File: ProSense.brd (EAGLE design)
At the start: 25.4 x 36.7 mm, 26 parts, among them U2 LPC1114FHI33/303, U4 MIC2505 3.3

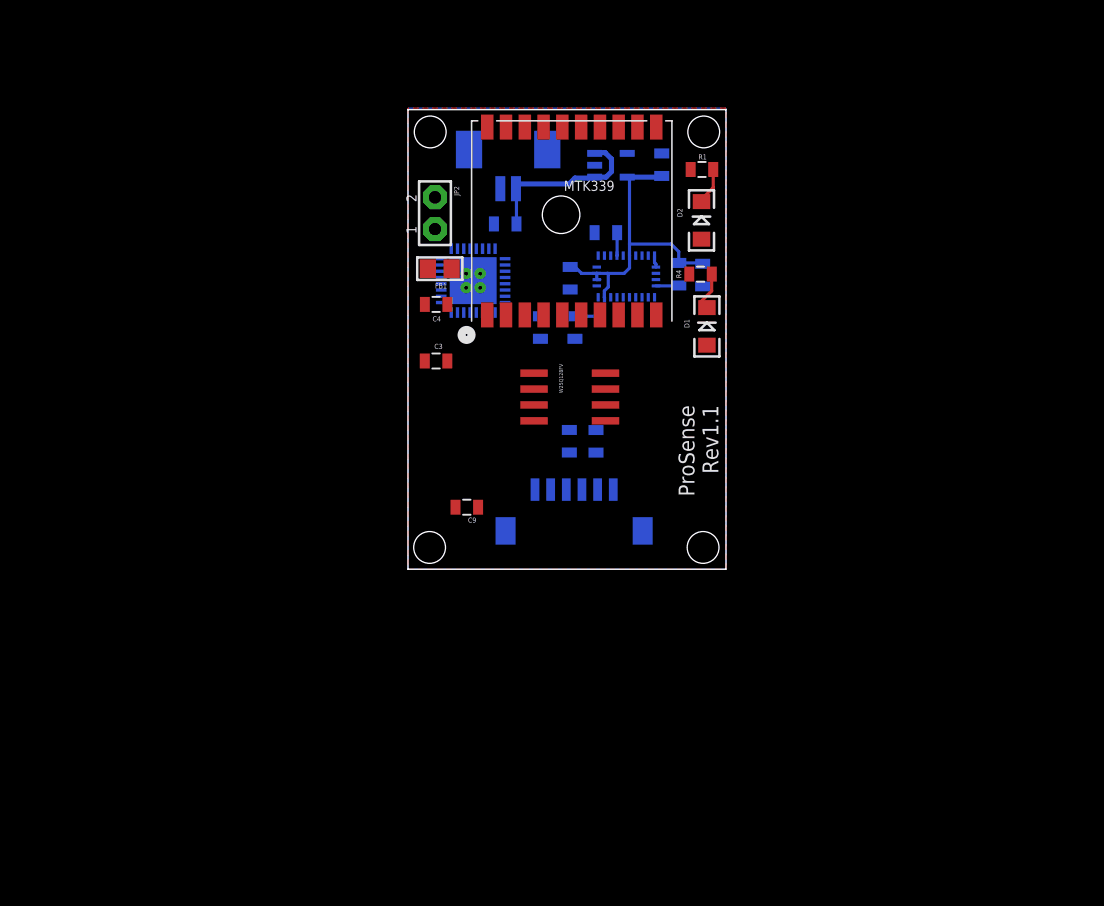
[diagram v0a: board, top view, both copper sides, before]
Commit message: Fixup
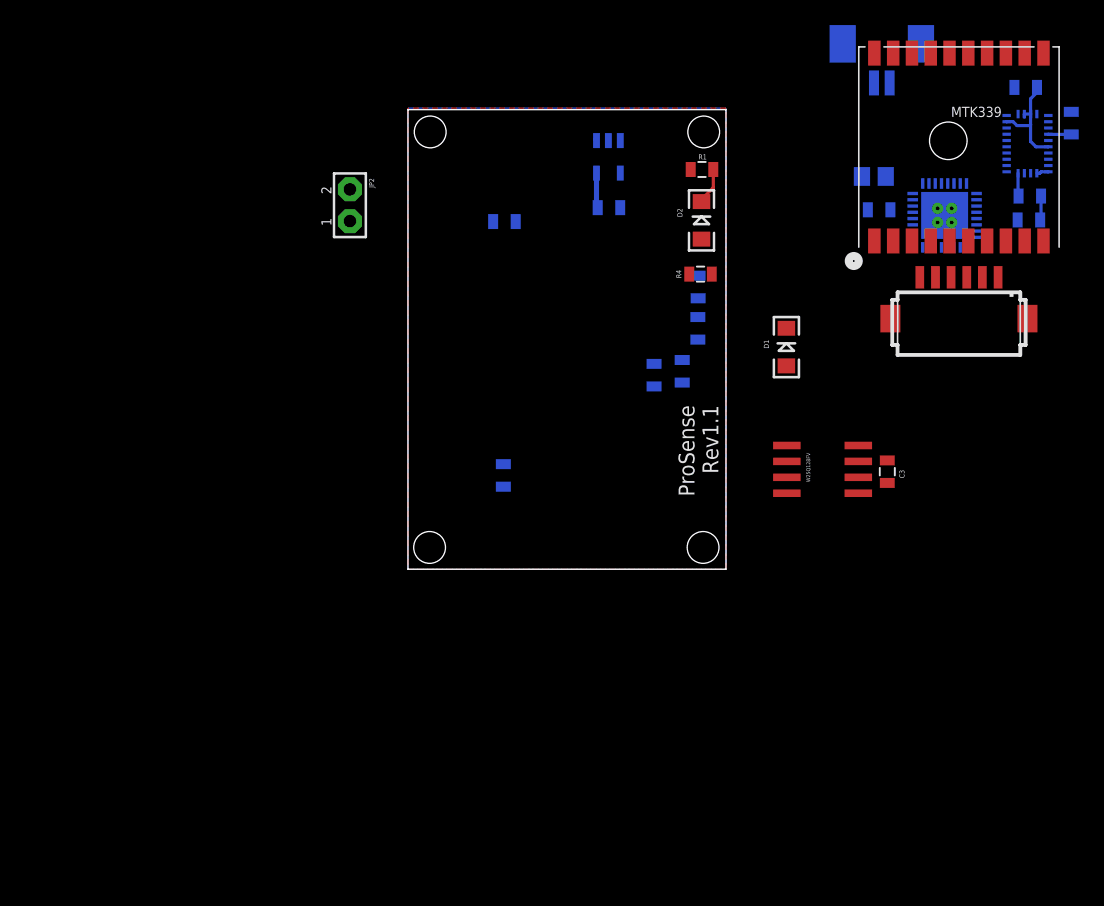
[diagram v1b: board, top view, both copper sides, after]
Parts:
- removed U2: LPC1114FHI33/303, NXP_60_26022015:SOT617-3
- added MCU: LPC1114FHI33/302, NXP_60_26022015:SOT617-3
- moved C6 39.4 mm to (84.9, 67.7), turned to 0 degrees
- moved C2 38.2 mm to (88.5, 64.8), turned to 270 degrees
- moved C3 37.1 mm to (73.8, 37.0), turned to 270 degrees
- moved C4 36.2 mm to (73.2, 57.9), flipped to the bottom
- moved FB1 35.4 mm to (72.8, 60.6), flipped to the bottom, turned to 180 degrees
- moved U$1 35.1 mm to (79.6, 51.6), flipped to the top
- moved BNO055 33.7 mm to (85.0, 63.2), turned to 0 degrees
- moved MTK339 31.5 mm to (79.6, 62.9)
- moved BAT_CON 31.0 mm to (73.4, 70.5)
- moved R7 28.7 mm to (85.2, 59.0), turned to 0 degrees
- moved R8 26.4 mm to (85.2, 57.1), turned to 180 degrees
- moved W25Q128FV 21.0 mm to (68.7, 37.2)
- moved C5 12.6 mm to (58.7, 48.5)
- moved C7 10.6 mm to (57.5, 45.0), turned to 270 degrees
- moved C1 10.4 mm to (58.7, 51.8), turned to 270 degrees
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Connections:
- net GND: now also MCU.33; no longer U2.33
- net ISP: now also MCU.3
- net LPC_RX: now also MCU.31; no longer U2.13
- net LPC_TX: now also MCU.32; no longer U2.14
- net RESET: now also MCU.2; no longer U2.2
- net SCL: now also MCU.10; no longer U2.10
- net SDA: now also MCU.11; no longer U2.11
- net VCC: now also MCU.29; no longer U2.29
- net VDD(IO): now also MCU.6; no longer U2.6
- net WS_CS: now also MCU.8
- net WS_DI: now also MCU.18
- net WS_DO: now also MCU.17
- net WS_SCK: now also MCU.15; no longer U2.15
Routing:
- net VCC: track 28.7 -> 13.7 mm
- net V_BATT: track 13.9 -> 0.10 mm
- net N$3: track 3.11 -> 0.00 mm

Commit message: Initial Revision for QFN packages
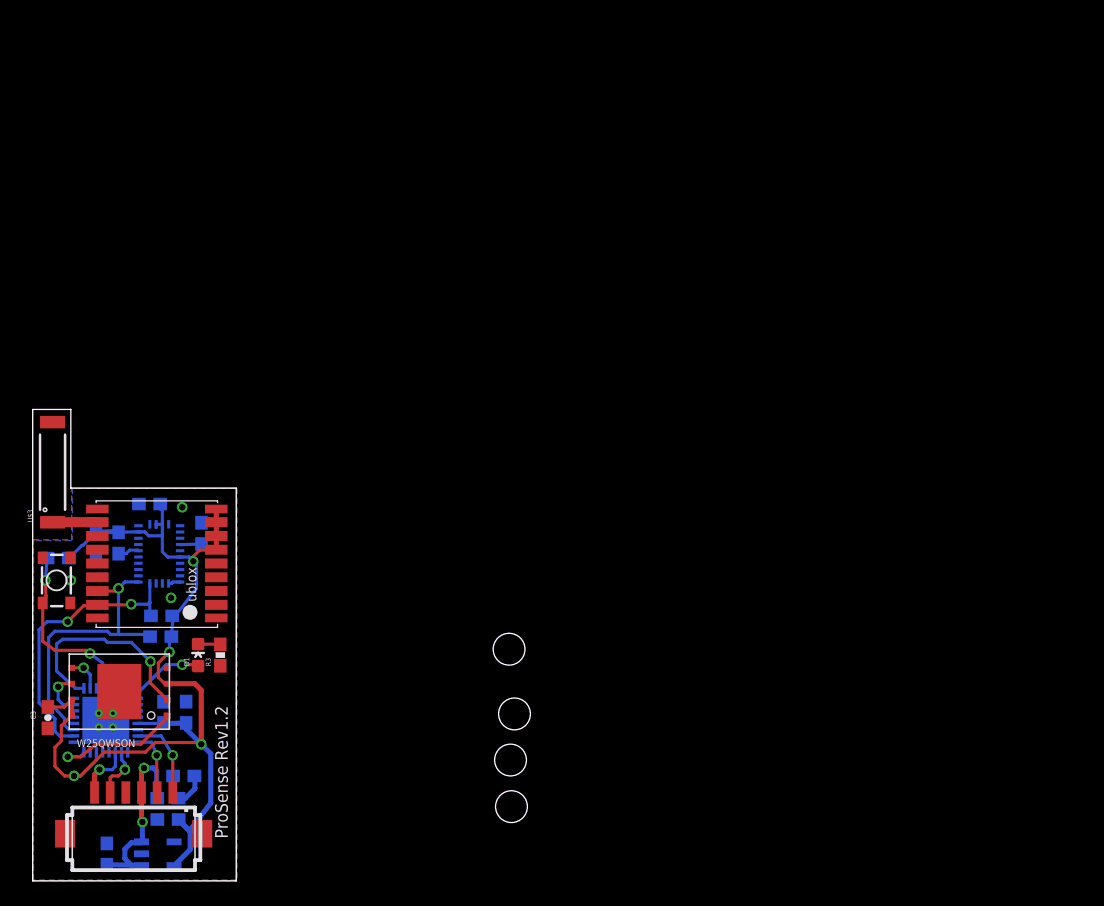
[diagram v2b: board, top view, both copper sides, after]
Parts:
- removed BAT_CON: 53261-02, con-molex:53261-02
- removed C4, C9: .1uF, SparkFun-Passives:0805
- removed D2: GREEN, SparkFun-LED:LED-1206
- removed FB1: GetValue, microbuilder:0805
- removed JP2: (no value), microbuilder:JUMPER2
- removed MTK339: (no value), adafruit:FGPMMOPA6H
- removed U4: MIC2505 3.3, SparkFun-PowerIC:SOT23-5
- removed W25Q128FV: (no value), Matts-Parts:8-SOIC
- added FRAME1: FRAME-LEDGER, SparkFun-Aesthetics:CREATIVE_COMMONS
- added MIC5205: 3.3, SparkFun-PowerIC:SOT23-5
- added R2: 1M, SparkFun-Passives:0603-RES
- added R3: 330, SparkFun-Passives:0603-RES
- added S2: SWITCH-MOMENTARY-2SMD-3, SparkFun-Electromechanical:TACTILE_SWITCH_SMD-3
- added U$2: UBLOX_MAX, Ava:UBLOX_MAX
- added U$3: ANTENNA2SMD3, SparkFun-RF:ANTENNA-CHIP4
- added W25QWSON: (no value), Matts-Parts:WSON-8-PAD
- C1, C14, C2, C3, C5, C6, C7, C8: device SparkFun-Passives:0805 -> SparkFun-Passives:0603-CAP
- C15: value .1uF -> 2.2uF; device SparkFun-Passives:0805 -> SparkFun-Passives:0603-CAP
- D1: value PURPLE -> (none); device SparkFun-LED:LED-1206 -> SparkFun-LED:LED-0603
- R1, R4: value 330 -> 10K; device SparkFun-Passives:0805 -> SparkFun-Passives:0603-RES
- R7, R8: device SparkFun-Passives:0805 -> SparkFun-Passives:0603-RES
- moved MCU 78.2 mm to (11.4, 17.1), turned to 90 degrees
- moved U$1 77.7 mm to (13.7, 10.5)
- moved C6 77.5 mm to (14.9, 34.4)
- moved R7 77.0 mm to (15.9, 25.5)
- moved R8 76.9 mm to (15.8, 23.8)
- moved C2 76.8 mm to (19.1, 32.1)
- moved BNO055 76.7 mm to (15.7, 30.4)
- moved C3 69.9 mm to (6.80, 17.4), turned to 90 degrees
- moved R1 65.9 mm to (16.4, 10.9), flipped to the bottom, turned to 0 degrees
- moved C15 60.2 mm to (16.4, 9.22), turned to 180 degrees
- moved C14 59.7 mm to (11.5, 6.46), turned to 270 degrees
- moved R4 56.1 mm to (7.62, 30.1), flipped to the bottom, turned to 180 degrees
- moved D1 53.0 mm to (18.8, 22.4), turned to 0 degrees
- moved C5 51.0 mm to (10.6, 31.3)
- moved C1 50.6 mm to (12.4, 31.3), turned to 90 degrees
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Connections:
- removed net GPS-LED: D2.A, MTK339.P$5
- removed net LPC_LED: D1.A
- removed net N$10: JP2.2, MTK339.P$1
- removed net N$3: D1.C, R4.2
- removed net N$4: C4.1, FB1.1, JP2.1
- removed net N$9: D2.C, R1.1
- removed net VDD(IO): MCU.6
- removed net V_BATT: BAT_CON.2, C14.2, U4.1, U4.3
- new net BAT_MONITOR: MCU.24, R1.1, R2.2
- new net BTN: MCU.20, R4.1, S2.4
- new net LED: D1.A, MCU.25
- new net N$1: U$2.11_RF_IN, U$3.SIG
- new net N$5: D1.C, R3.2
- new net VIN: C14.2, MIC5205.1, MIC5205.3, R1.2, U$1.P$3
- net GND: now also MIC5205.2, R2.1, R3.1, S2.1, U$2.10_GND, U$2.12_GND, U$2.1_GND, W25QWSON.4; no longer BAT_CON.1, C4.2, C9.1, MTK339.P$12, MTK339.P$19, MTK339.P$3, MTK339.P$8, R1.2, R4.1, U4.2, W25Q128FV.4
- net LPC_RX: no longer MTK339.P$9
- net LPC_TX: no longer MTK339.P$10
- net SCL: now also U$2.17_SCL2
- net SDA: now also U$2.16_SDA2
- net VCC: now also MCU.6, MIC5205.5, R4.2, U$2.6_V_BCKP, U$2.7_VCC_IO, U$2.8_VCC, U$2.9_V_RESET, W25QWSON.3, W25QWSON.7, W25QWSON.8; no longer C9.2, FB1.2, U$1.P$3, U4.5, W25Q128FV.3, W25Q128FV.7, W25Q128FV.8
- net WS_CS: now also W25QWSON.1; no longer W25Q128FV.1
- net WS_DI: now also W25QWSON.5; no longer W25Q128FV.5
- net WS_DO: now also W25QWSON.2; no longer W25Q128FV.2
- net WS_SCK: now also W25QWSON.6; no longer W25Q128FV.6
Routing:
- net VCC: track 13.7 -> 84.4 mm, vias 0 -> 4
- net SDA: track 0.00 -> 24.2 mm, vias 0 -> 1
- net SCL: track 1.84 -> 22.7 mm, vias 0 -> 2
- net WS_DO: track 0.00 -> 16.8 mm, vias 0 -> 1
- net VIN: track 0.00 -> 16.0 mm, vias 0 -> 2
- net BTN: track 0.00 -> 14.1 mm, vias 0 -> 2
- net WS_CS: track 0.00 -> 10.8 mm, vias 0 -> 1
- net LPC_RX: track 0.00 -> 6.65 mm, vias 0 -> 1
- net LED: track 0.00 -> 6.23 mm, vias 0 -> 1
- net LPC_TX: track 0.00 -> 5.21 mm, vias 0 -> 1
- net ISP: track 0.00 -> 4.51 mm, vias 0 -> 1
- net RESET: track 0.00 -> 4.12 mm, vias 0 -> 1
- net WS_SCK: track 0.00 -> 3.63 mm, vias 0 -> 1
- net N$1: track 0.00 -> 3.58 mm
- net N$9: track 2.95 -> 0.00 mm
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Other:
- board size 25.4 x 36.7 mm -> 16.3 x 37.7 mm
- board text added: "ProSense Rev1.2"
- board text removed: "ProSense Rev1.1"
